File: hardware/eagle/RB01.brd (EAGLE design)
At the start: 50 x 31 mm, 10 parts, among them J1 CON_TERMINAL_BLOCK_03-5MM, J2 CON_TERMINAL_BLOCK_02-5MM, K1 JS-M1A-12V-5, Q1 BC337

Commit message: Magic Smoke logo
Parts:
- added U$2: (no value), SparkFun:OSHW-LOGO-S
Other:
- board text added: "/Users/thomasprice/Documents/eagle/logo/Magic_Smoke_logo.bmp"

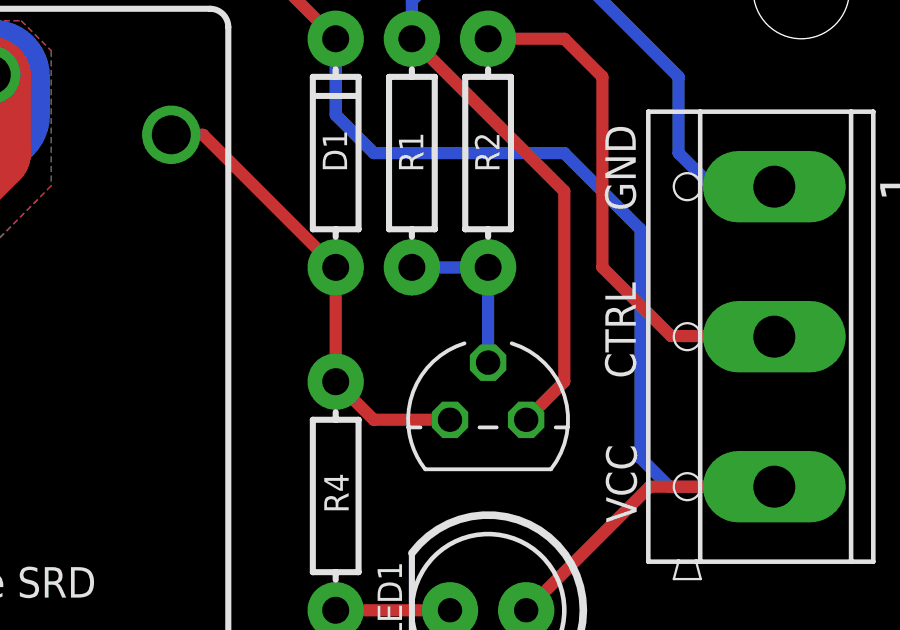
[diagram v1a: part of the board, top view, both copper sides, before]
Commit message: tweak gerbers
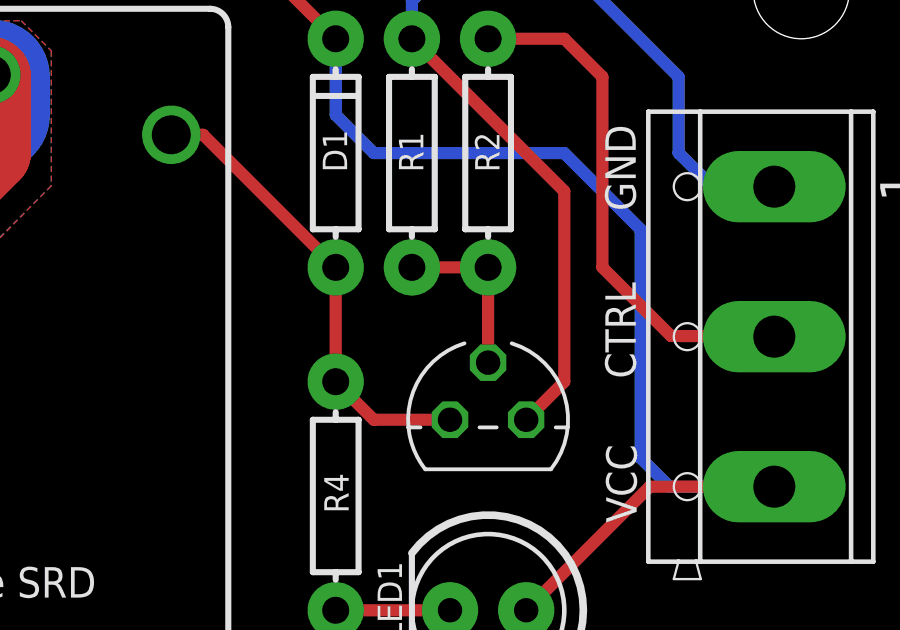
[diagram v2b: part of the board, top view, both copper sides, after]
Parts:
- moved U$2 1.30 mm to (19.1, 5.59)
